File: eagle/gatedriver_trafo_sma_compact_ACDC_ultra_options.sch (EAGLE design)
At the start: 98 parts, among them K1 G5V-2, X4 BU-SMA-V

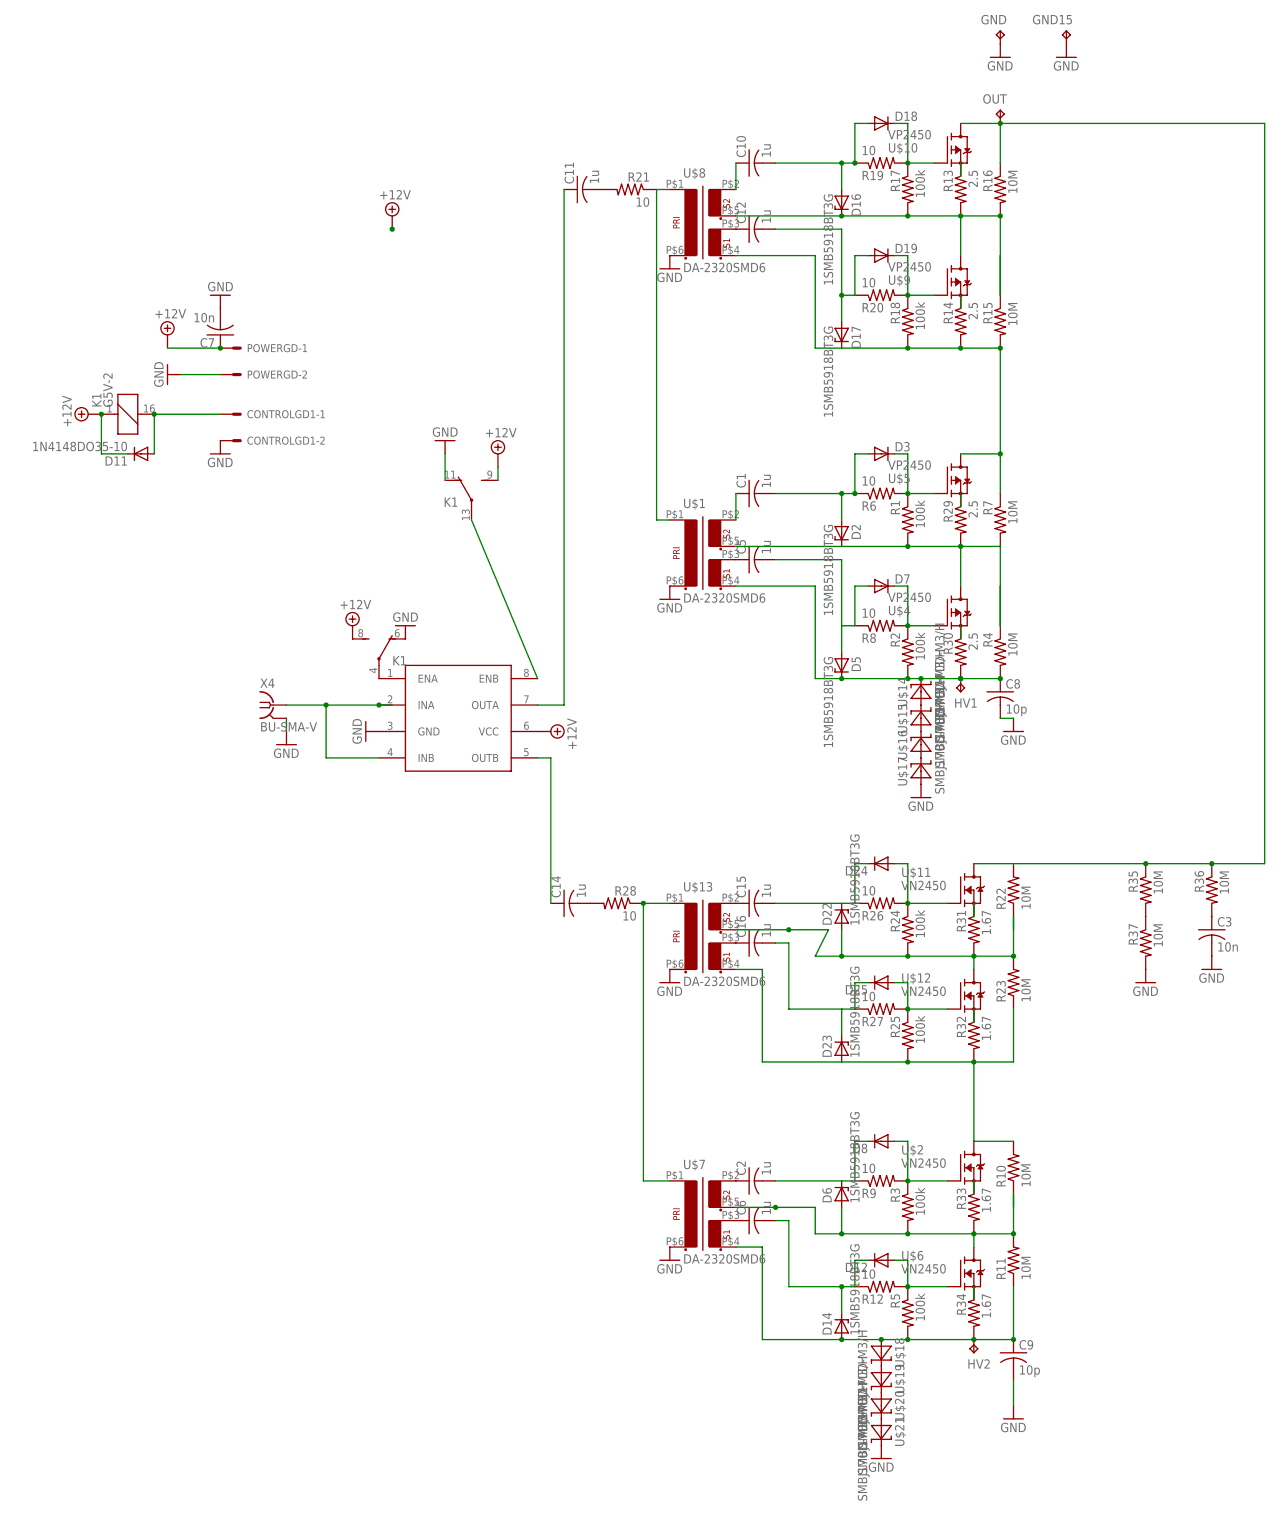
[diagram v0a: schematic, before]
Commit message: gd mods
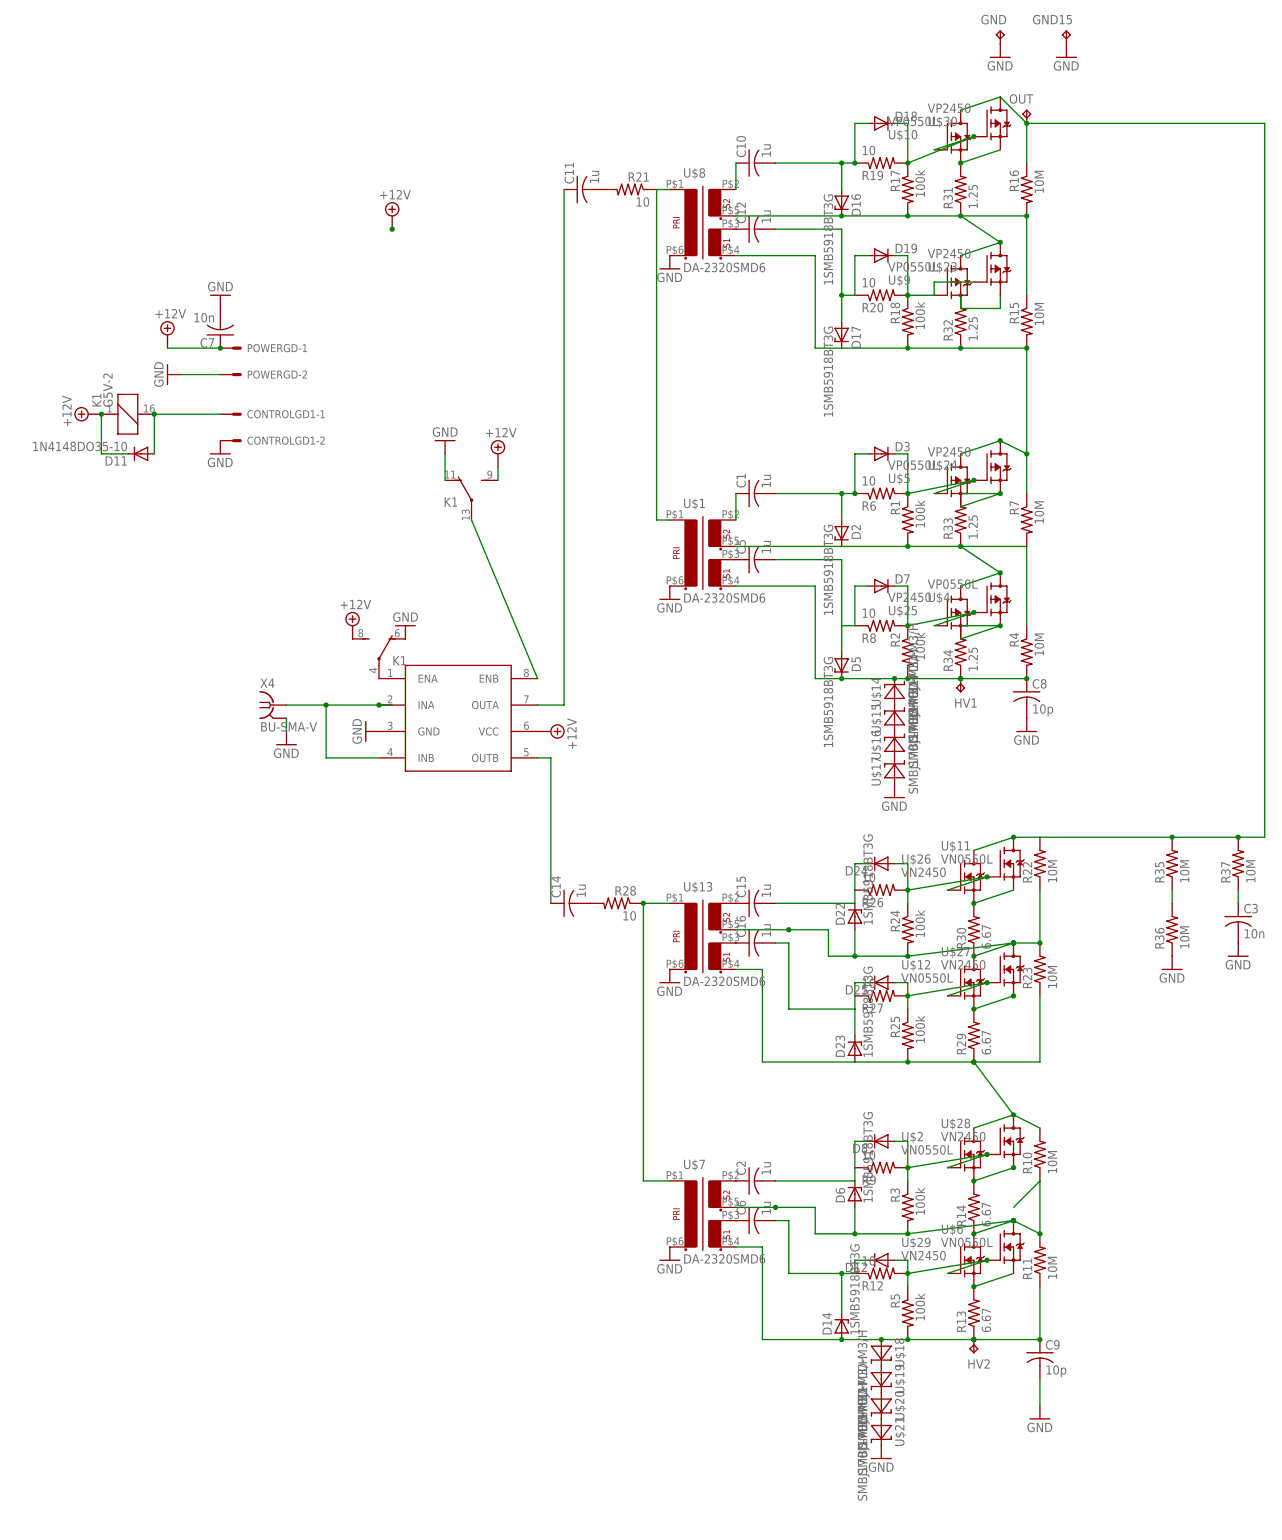
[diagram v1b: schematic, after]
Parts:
- added U$23, U$24, U$25, U$30: VP2450, transistor-fet:VP2450
- added U$26, U$27, U$28, U$29: VN2450, transistor-fet:VN2450
- R13, R14, R29, R30: value 2.5 -> 6.67
- R31, R32, R33, R34: value 1.67 -> 1.25
- U$10, U$4, U$5, U$9: value VP2450 -> VP0550L; device transistor-fet:VP2450 -> transistor-fet:VP0550L
- U$11, U$12, U$2, U$6: value VN2450 -> VN0550L; device transistor-fet:VN2450 -> transistor-fet:VN0550L
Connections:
- removed net N$57 (its old number): R14.1, U$9.S
- new net N$45: C3.1, R37.1
- net GND: now also R36.1; no longer R37.2
- net N$11: now also U$29.G
- net N$12: now also U$25.G
- net N$13: now also R14.1, U$29.D; no longer R33.2
- net N$17: now also R34.1; no longer R30.2
- net N$18: now also R33.1, U$25.D; no longer R29.2
- net N$19: now also R30.2, U$26.S; no longer R31.1
- net N$20: now also R34.2, U$25.S, U$4.S; no longer R32.1, U$12.S
- net N$21: now also R33.2, U$24.S, U$5.S; no longer R33.1, U$2.S
- net N$24: now also R13.1; no longer R34.2
- net N$251: now also U$28.G
- net N$26: now also R35.2, R37.2, U$26.D, U$30.D; no longer R35.1, R36.1
- net N$3: now also R13.2, U$29.S, U$6.S; no longer R13.1, U$10.S
- net N$31: now also R31.2, U$10.S, U$30.S; no longer R34.1, U$6.S
- net N$32: now also R32.1, U$24.D; no longer R14.2
- net N$33: now also R31.1, U$23.D; no longer R13.2
- net N$34: now also U$30.G
- net N$36: now also U$23.G
- net N$39: now also R32.2, U$23.S, U$9.S; no longer C3.1, R36.2
- net N$44: now also R35.1, R36.2; no longer R35.2, R37.1
- net N$46: now also R30.1, U$27.D; no longer R31.2
- net N$47: now also U$27.G
- net N$50: now also U$26.G
- net N$51: now also R29.1, U$28.D; no longer R32.2
- net N$6: now also R14.2, U$2.S, U$28.S; no longer R30.1, U$4.S
- net N$8: now also U$24.G
- net N$9: now also R29.2, U$12.S, U$27.S; no longer R29.1, U$5.S
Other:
- moved on the sheet: C3, C8, C9, D22, D23, D6, OUT, R10, R11, R12, R13, R14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
